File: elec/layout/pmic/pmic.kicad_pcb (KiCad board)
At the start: 2 copper layers, 24 parts, among them U1 _PCA9450AAHNY

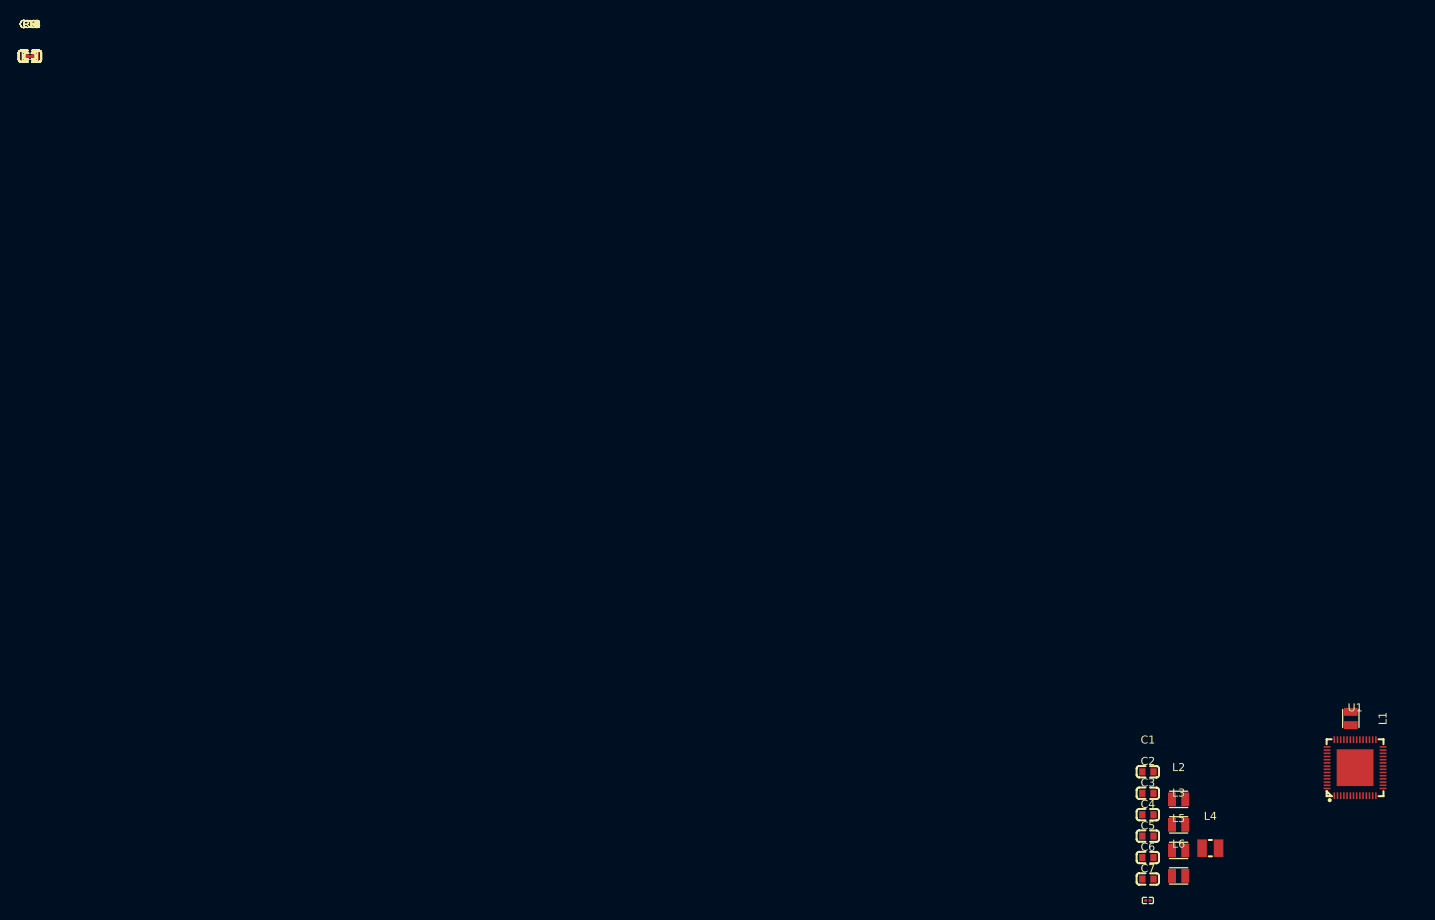
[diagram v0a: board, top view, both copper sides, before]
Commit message: pmic layout file
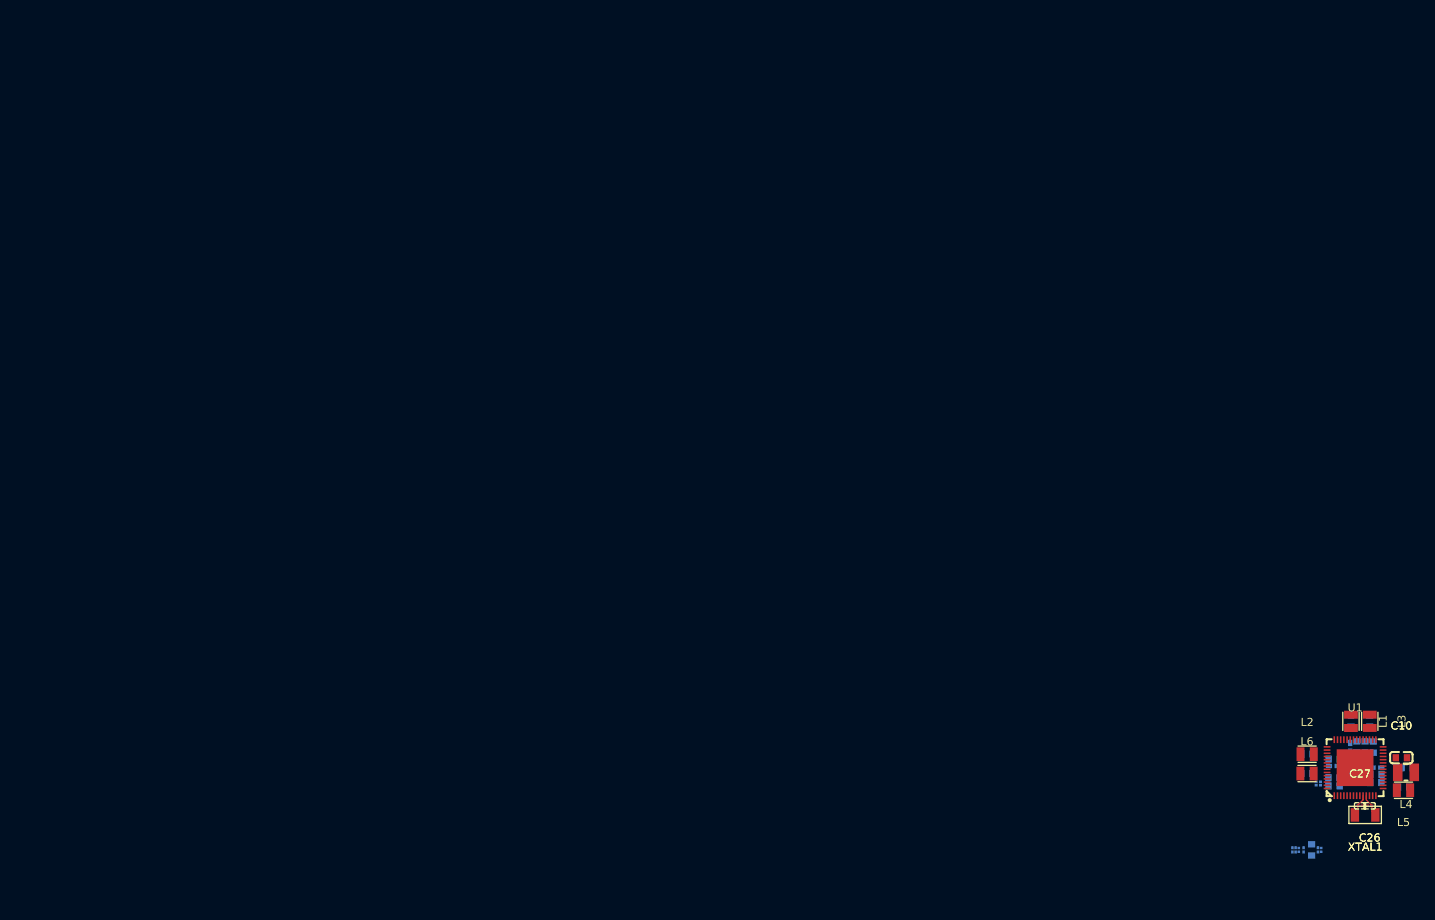
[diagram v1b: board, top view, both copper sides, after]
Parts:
- added C16: 2.2µF ±20% 10V X5R, lcsc:C0402, B.Cu at (168.4, 88.9)
- added C17: 2.2µF ±20% 10V X5R, lcsc:C0402, B.Cu at (162.9, 88.7)
- added C18: 10µF ±10% 10V X5R, lcsc:C0603, B.Cu at (163.0, 91.2)
- added C19: 10µF ±10% 10V X5R, lcsc:C0603, B.Cu at (163.0, 90.2)
- added C20: 10µF ±10% 10V X5R, lcsc:C0603, B.Cu at (166.9, 86.3)
- added C21: 10µF ±10% 10V X5R, lcsc:C0603, B.Cu at (167.9, 86.3)
- added C22: 10µF ±10% 10V X5R, lcsc:C0603, B.Cu at (168.2, 90.8)
- added C23: 10µF ±10% 10V X5R, lcsc:C0603, B.Cu at (168.2, 89.8)
- added C24: 10µF ±10% 10V X5R, lcsc:C0603, B.Cu at (163.0, 87.9)
- added C25: 2.2µF ±20% 10V X5R, lcsc:C0402, B.Cu at (165.0, 86.4)
- added C26: 10pF ±5% 50V C0G, lcsc:C0201, F.Cu at (167.5, 93.7)
- added C27: 10pF ±5% 50V C0G, lcsc:C0201, F.Cu at (166.3, 93.7)
- added XTAL1: Crystal, lcsc:OSC-SMD_L3.2-W1.5, F.Cu at (166.9, 94.8)
- C1, C11, C12, C13, C14, C2, C3, C4, C5, C6, C7, C8, C9: moved to B.Cu
- C15: value 82nF ±5% 25V X7R -> 10µF ±10% 10V X5R; moved to B.Cu
- R1: value 10kΩ ±1% 62.5mW -> 10kΩ ±1% 50mW; footprint lcsc:R0402 -> lcsc:R0201; moved to B.Cu
- R2: value 750mΩ ±5% 100mW -> 1.5Ω ±5% 50mW; footprint lcsc:R0603 -> lcsc:R0201; moved to B.Cu
- moved C10 192.6 mm to (171.4, 87.7)
- moved R2 189.4 mm to (161.4, 99.2), turned to -90 degrees
- moved C13 189.1 mm to (161.0, 99.2), turned to -90 degrees
- moved C9 188.4 mm to (160.2, 99.2), turned to -90 degrees
- moved C14 187.6 mm to (159.2, 99.2), turned to -90 degrees
- moved R1 187.1 mm to (158.6, 99.2), turned to -90 degrees
- moved C15 187.0 mm to (165.9, 86.3), turned to -90 degrees
- moved C8 186.7 mm to (158.2, 99.2), turned to -90 degrees
- moved C12 186.4 mm to (157.8, 99.2), turned to -90 degrees
- moved C11 184.8 mm to (161.0, 90.7), turned to 180 degrees
- moved C4 33.5 mm to (172.1, 88.9), turned to 180 degrees
- moved C5 33.2 mm to (171.7, 91.3), turned to 180 degrees
- moved C3 30.1 mm to (167.5, 83.1), turned to -90 degrees
- moved L5 29.1 mm to (171.7, 91.8), turned to 180 degrees
- moved L3 27.2 mm to (167.5, 83.1), turned to -90 degrees
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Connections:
- net *3A58.pmic-lv renamed *3B78.pmic-lv
- net *3A58.pmic-net-1 renamed *3B78.pmic-net-3
- net *3A58.pmic.VDD_PHY_1V2-lv renamed *3B78.pmic.VDD_PHY_1V2-lv
- net *3A58.pmic.pmic-net renamed *3B78.pmic.pmic-net
- net signal renamed RTC_RESET_B
- C10 pad 1: *3A58.pmic-net-0 -> VCC_3V3
- C11 pad 2: *3A58.pmic.VDDA_1V8-lv -> GND
- C12 pad 2: *3A58.pmic.VDD_PHY_0V9-lv -> GND
- C14 pad 2: *3A58.pmic.VDD_SNVS_0V8-lv -> GND
- C7 pad 2: *3A58.pmic.NVCC_SD2-lv -> GND
- C8 pad 2: *3A58.pmic.NVCC_SNVS_1V8-lv -> GND
- R2 pad 2: *3A58.pmic-net-0 -> *3B78.pmic-net-2
- U1 pad 10: xtal_in -> *3B78.pmic-net-1
- U1 pad 11: xtal_out -> *3B78.pmic-net-0
- U1 pad 12: sw_en -> *3B78.pmic-net-2
- U1 pad 23: *3A58.pmic-net-0 -> VCC_3V3
- U1 pad 43: GND -> buck_agnd
- U1 pad 5: GND -> agnd
- U1 pad 57: GND -> ep
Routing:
- net *3B78.pmic-net-0: track 0.00 -> 2.88 mm
- net *3B78.pmic-net-1: track 0.00 -> 2.83 mm

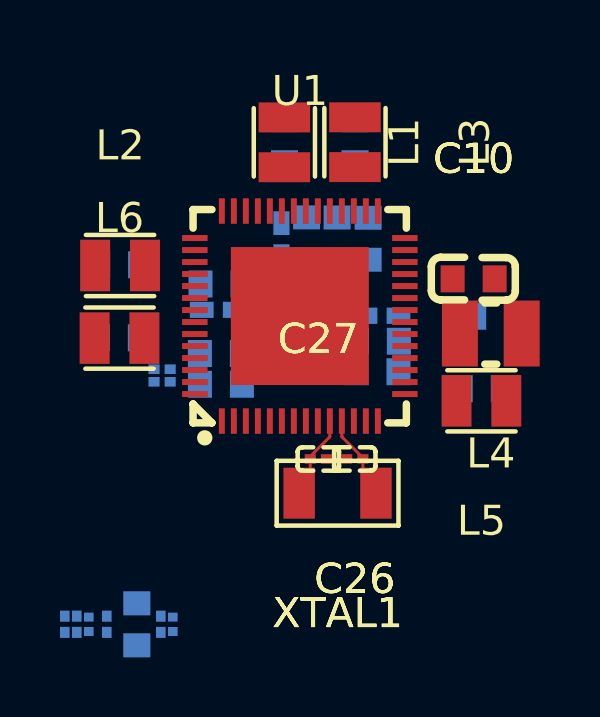
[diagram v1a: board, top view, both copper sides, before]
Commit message: Layout 90% complete
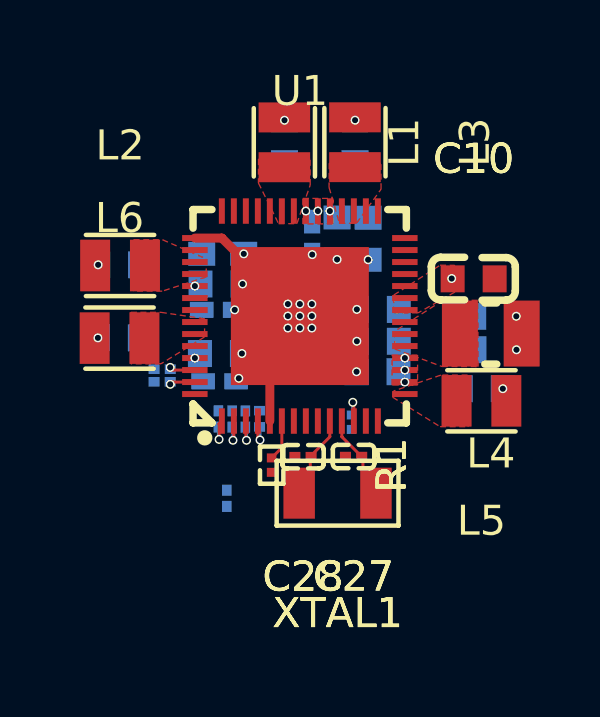
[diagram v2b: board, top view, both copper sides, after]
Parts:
- added C28: 10pF ±5% 50V C0G, lcsc:C0201, F.Cu at (165.7, 93.6)
- C15: value 10µF ±10% 10V X5R -> 1µF ±20% 6.3V X5R; footprint lcsc:C0603 -> lcsc:C0201
- C16, C25: value 2.2µF ±20% 10V X5R -> 10µF ±10% 10V X5R; footprint lcsc:C0402 -> lcsc:C0603
- C18: value 10µF ±10% 10V X5R -> 2.2µF ±20% 10V X5R; footprint lcsc:C0603 -> lcsc:C0402
- C26: value 10pF ±5% 50V C0G -> 2.2µF ±20% 10V X5R; footprint lcsc:C0201 -> lcsc:C0402; moved to B.Cu
- R1: moved to F.Cu
- moved C9 15.1 mm to (172.2, 90.0), turned to 180 degrees
- moved R2 8.99 mm to (167.4, 92.5), turned to 90 degrees
- moved C8 8.85 mm to (163.8, 92.4), turned to 90 degrees
- moved C12 8.55 mm to (162.9, 92.4), turned to 90 degrees
- moved R1 8.08 mm to (164.7, 93.9)
- moved C14 8.02 mm to (163.4, 92.4), turned to 90 degrees
- moved C26 7.50 mm to (166.0, 86.3), turned to -90 degrees
- moved C15 6.22 mm to (164.3, 92.4), turned to 90 degrees
- moved C13 4.74 mm to (163.2, 95.0)
- moved C25 2.01 mm to (163.1, 86.9), turned to 0 degrees
- moved C27 1.18 mm to (167.4, 93.6), turned to 180 degrees
- moved C16 0.25 mm to (168.2, 88.7)
- moved C18 0.11 mm to (163.0, 91.1)
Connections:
- net *3B78.pmic-net-2 renamed *3AE8.pmic-net-0
- net *3B78.pmic-net-3 renamed *3AE8.pmic-net-2
- net *3B78.pmic.VDD_PHY_1V2-lv renamed lv
- net *3B78.pmic.pmic-net renamed *3AE8.pmic.pmic-net
- net VDD_1V8_SW renamed VDD_3V3_SW
- C10 pad 2: *3B78.pmic-lv -> GND
- C15 pad 1: VSYS_5V -> *3AE8.pmic-net-4
- C26 pad 1: *3B78.pmic-net-0 -> VSYS_5V
- C27 pad 1: *3B78.pmic-net-1 -> *3AE8.pmic-net-1
- U1 pad 10: *3B78.pmic-net-1 -> *3AE8.pmic-net-3
- U1 pad 11: *3B78.pmic-net-0 -> *3AE8.pmic-net-1
- U1 pad 14: buck5fb -> VDD_1V8
- U1 pad 21: VDD_1V8 -> VCC_3V3
- U1 pad 4: vint -> *3AE8.pmic-net-4
- U1 pad 43: buck_agnd -> GND
- U1 pad 5: agnd -> GND
- U1 pad 53: vsys -> VSYS_5V
- U1 pad 57: ep -> GND
- XTAL1 pad 1: *3B78.pmic-net-0 -> *3AE8.pmic-net-1
- XTAL1 pad 2: *3B78.pmic-net-1 -> *3AE8.pmic-net-3
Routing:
- net GND: track 0.00 -> 8.49 mm, vias 0 -> 20
- net *3B78.pmic-net-0: track 2.88 -> 0.00 mm
- net *3AE8.pmic-net-0: track 0.00 -> 2.88 mm
- net *3B78.pmic-net-1: track 2.83 -> 0.00 mm
- net *3AE8.pmic-net-2: track 0.00 -> 2.83 mm
- net *3AE8.pmic-net-4: track 0.00 -> 1.37 mm
- net VCC_3V3: track 0.00 -> 1.30 mm, vias 0 -> 3
- net NVCC_SNVS_1V8: track 0.00 -> 1.10 mm, vias 0 -> 1
- net VDD_SNVS_0V8: track 0.00 -> 1.10 mm, vias 0 -> 1
- net *3AE8.pmic-net-1: track 0.00 -> 1.10 mm, vias 0 -> 1
- net *3AE8.pmic-net-3: track 0.00 -> 1.08 mm, vias 0 -> 1
- net VDD_PHY_0V9: track 0.00 -> 1.07 mm, vias 0 -> 1
- net VDDA_1V8: track 0.00 -> 0.86 mm, vias 0 -> 1
- net NVCC_SD2: track 0.00 -> 0.85 mm, vias 0 -> 1
- net VDD_1V8: track 0.00 -> 0.45 mm, vias 0 -> 1
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- added copper zone on F.Cu, net VCC_3V3
- added copper zone on F.Cu, net VDDA_1V8_SW
- added copper zone on F.Cu, net VDD_3V3_SW
- added copper zone on F.Cu, net VDD_ARM_0V9_SW
- added copper zone on F.Cu, net VDD_PHY_0V9_SW
- added copper zone on F.Cu, net VDD_SOC_0V8_SW
- added copper zone on F.Cu, net VSYS_5V
